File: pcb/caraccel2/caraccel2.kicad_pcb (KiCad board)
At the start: 2 copper layers, 100 x 100 mm, 11 parts, among them J1 LESP, J2 RESP

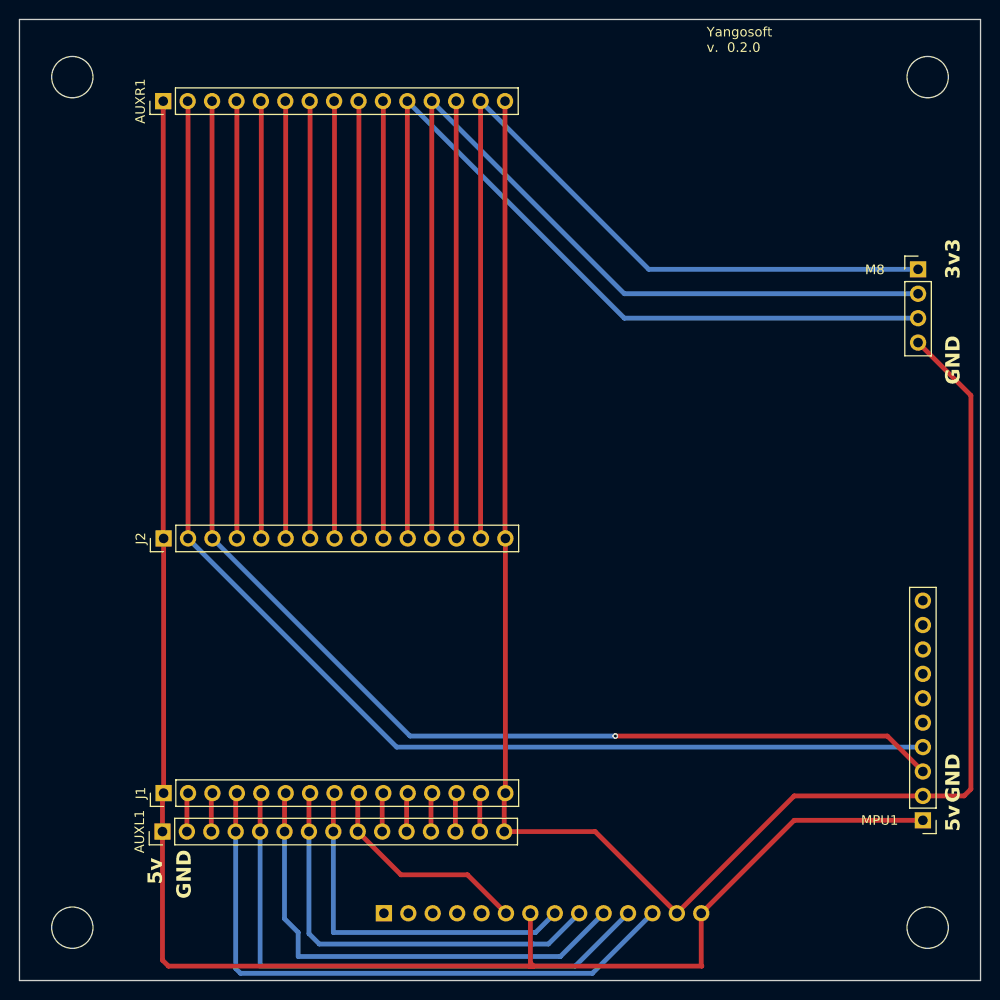
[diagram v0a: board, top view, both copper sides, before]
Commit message: New FreeRTOS and LVGL version
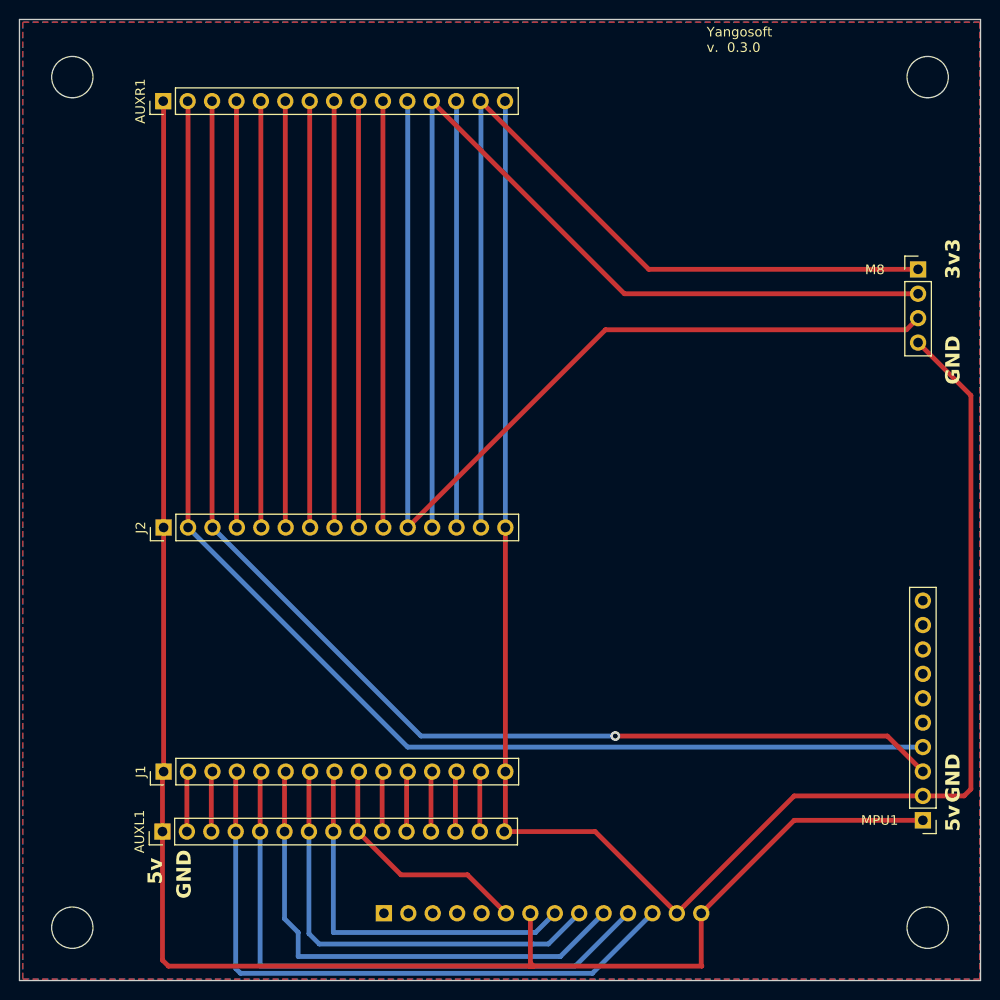
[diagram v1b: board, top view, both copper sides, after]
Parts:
- moved J1 2.24 mm to (116.0, 111.8)
- moved J2 1.14 mm to (116.0, 86.4)
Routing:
- net GND: track 186.3 -> 188.7 mm
- net /CS: track 64.5 -> 66.7 mm
- net /RST: track 58.7 -> 60.9 mm
- net /MOSI: track 44.6 -> 46.8 mm
- net Net-(AUXL1-Pin_3): track 4.05 -> 6.29 mm
- net Net-(AUXL1-Pin_14): track 4.05 -> 6.29 mm
- net Net-(AUXL1-Pin_12): track 4.05 -> 6.29 mm
- net Net-(AUXL1-Pin_11): track 4.05 -> 6.29 mm
- net Net-(AUXL1-Pin_10): track 4.05 -> 6.29 mm
- net Net-(AUXL1-Pin_13): track 4.05 -> 6.29 mm
- net /MISO: track 23.0 -> 25.2 mm
- net /SLK: track 38.4 -> 40.7 mm
- net /DC: track 51.3 -> 53.5 mm
- net /RX: track 108.0 -> 106.5 mm
- net /TX: track 104.4 -> 103.3 mm
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- added copper zone on F.Cu, net +5V
- added copper zone on B.Cu, net GND
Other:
- board text added: "Yangosoft v. 0.3.0"
- board text removed: "Yangosoft v. 0.2.0"
